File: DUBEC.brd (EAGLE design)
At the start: 40 x 21.4 mm, 72 parts

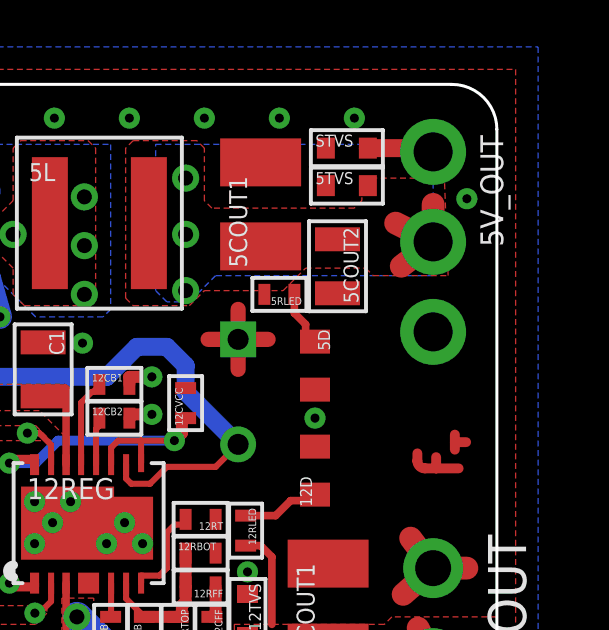
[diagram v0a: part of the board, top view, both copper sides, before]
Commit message: Tweaks
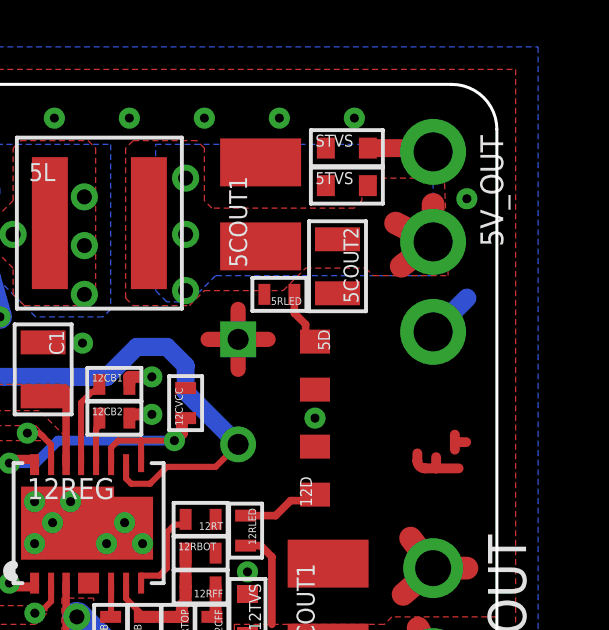
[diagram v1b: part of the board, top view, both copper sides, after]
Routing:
- net GND: track 34.1 -> 35.7 mm
- net 5V: track 44.4 -> 43.5 mm
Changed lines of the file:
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@@
 <grid distance="0.125" unitdist="mm" unit="mm" style="lines" multiple="8" display="yes" altdistance="0.0625" altunitdist="mm" altunit="mm"/>
 <layers>
-<layer number="1" name="Top" color="2" fill="1" visible="yes" active="yes"/>
+<layer number="1" name="Top" color="2" fill="1" visible="no" active="yes"/>
 <layer number="2" name="Route2" color="9" fill="1" visible="no" active="yes"/>
 <layer number="3" name="Route3" color="4" fill="3" visible="no" active="no"/>
 <layer number="14" name="Route14" color="1" fill="6" visible="no" active="no"/>
-<layer number="15" name="Route15" color="14" fill="1" visible="yes" active="yes"/>
+<layer number="15" name="Route15" color="14" fill="1" visible="no" active="yes"/>
 <layer number="16" name="Bottom" color="5" fill="1" visible="yes" active="yes"/>
 <layer number="17" name="Pads" color="10" fill="1" visible="yes" active="yes"/>
@@
 <layer number="20" name="Dimension" color="15" fill="1" visible="yes" active="yes"/>
 <layer number="21" name="tPlace" color="15" fill="1" visible="no" active="yes"/>
-<layer number="22" name="bPlace" color="7" fill="1" visible="no" active="yes"/>
-<layer number="23" name="tOrigins" color="15" fill="1" visible="yes" active="yes"/>
+<layer number="22" name="bPlace" color="7" fill="1" visible="yes" active="yes"/>
+<layer number="23" name="tOrigins" color="15" fill="1" visible="no" active="yes"/>
 <layer number="24" name="bOrigins" color="15" fill="1" visible="yes" active="yes"/>
 <layer number="25" name="tNames" color="7" fill="1" visible="no" active="yes"/>
@@
 <layer number="27" name="tValues" color="7" fill="1" visible="no" active="yes"/>
 <layer number="28" name="bValues" color="7" fill="1" visible="no" active="yes"/>
-<layer number="29" name="tStop" color="4" fill="1" visible="yes" active="yes"/>
+<layer number="29" name="tStop" color="4" fill="1" visible="no" active="yes"/>
 <layer number="30" name="bStop" color="7" fill="6" visible="yes" active="yes"/>
-<layer number="31" name="tCream" color="7" fill="4" visible="yes" active="yes"/>
+<layer number="31" name="tCream" color="7" fill="4" visible="no" active="yes"/>
 <layer number="32" name="bCream" color="7" fill="5" visible="yes" active="yes"/>
-<layer number="33" name="tFinish" color="6" fill="3" visible="yes" active="yes"/>
+<layer number="33" name="tFinish" color="6" fill="3" visible="no" active="yes"/>
 <layer number="34" name="bFinish" color="6" fill="6" visible="yes" active="yes"/>
-<layer number="35" name="tGlue" color="7" fill="4" visible="yes" active="yes"/>
+<layer number="35" name="tGlue" color="7" fill="4" visible="no" active="yes"/>
 <layer number="36" name="bGlue" color="7" fill="5" visible="yes" active="yes"/>
-<layer number="37" name="tTest" color="7" fill="1" visible="yes" active="yes"/>
+<layer number="37" name="tTest" color="7" fill="1" visible="no" active="yes"/>
 <layer number="38" name="bTest" color="7" fill="1" visible="yes" active="yes"/>
-<layer number="39" name="tKeepout" color="4" fill="11" visible="yes" active="yes"/>
+<layer number="39" name="tKeepout" color="4" fill="11" visible="no" active="yes"/>
 <layer number="40" name="bKeepout" color="1" fill="11" visible="yes" active="yes"/>
-<layer number="41" name="tRestrict" color="14" fill="10" visible="yes" active="yes"/>
+<layer number="41" name="tRestrict" color="14" fill="10" visible="no" active="yes"/>
 <layer number="42" name="bRestrict" color="1" fill="10" visible="yes" active="yes"/>
 <layer number="43" name="vRestrict" color="2" fill="10" visible="no" active="yes"/>
 <layer number="44" name="Drills" color="7" fill="1" visible="no" active="yes"/>
-<layer number="45" name="Holes" color="7" fill="1" visible="no" active="yes"/>
+<layer number="45" name="Holes" color="7" fill="1" visible="yes" active="yes"/>
 <layer number="46" name="Milling" color="3" fill="1" visible="no" active="yes"/>
 <layer number="47" name="Measures" color="7" fill="1" visible="yes" active="yes"/>
-<layer number="48" name="Document" color="7" fill="1" visible="no" active="yes"/>
+<layer number="48" name="Document" color="7" fill="1" visible="yes" active="yes"/>
 <layer number="49" name="Reference" color="7" fill="1" visible="no" active="yes"/>
 <layer number="50" name="dxf" color="7" fill="1" visible="no" active="no"/>
 <layer number="51" name="tDocu" color="7" fill="1" visible="no" active="yes"/>
-<layer number="52" name="bDocu" color="7" fill="1" visible="no" active="yes"/>
+<layer number="52" name="bDocu" color="7" fill="1" visible="yes" active="yes"/>
 <layer number="53" name="tGND_GNDA" color="7" fill="9" visible="no" active="no"/>
 <layer number="54" name="bGND_GNDA" color="1" fill="9" visible="no" active="no"/>
@@
 <layer number="100" name="Muster" color="7" fill="1" visible="no" active="no"/>
 <layer number="101" name="Patch_Top" color="12" fill="4" visible="no" active="yes"/>
-<layer number="102" name="tPolarity" color="7" fill="1" visible="yes" active="yes"/>
+<layer number="102" name="tPolarity" color="7" fill="1" visible="no" active="yes"/>
 <layer number="103" name="tMap" color="7" fill="1" visible="no" active="yes"/>
 <layer number="104" name="Name" color="16" fill="1" visible="no" active="yes"/>
-<layer number="105" name="tPlate" color="7" fill="1" visible="yes" active="yes"/>
+<layer number="105" name="tPlate" color="7" fill="1" visible="no" active="yes"/>
 <layer number="106" name="bPlate" color="7" fill="1" visible="no" active="yes"/>
-<layer number="107" name="tLabels" color="15" fill="1" visible="yes" active="yes"/>
+<layer number="107" name="tLabels" color="15" fill="1" visible="no" active="yes"/>
 <layer number="108" name="tplace-old" color="10" fill="1" visible="no" active="yes"/>
 <layer number="109" name="ref-old" color="11" fill="1" visible="no" active="yes"/>
@@
 <wire x1="36.5" y1="1" x2="36.75" y2="0.75" width="0.254" layer="1"/>
 <wire x1="36.75" y1="0.75" x2="38.75" y2="0.75" width="0.254" layer="1"/>
+<wire x1="37.875" y1="13.125" x2="39" y2="14.25" width="0.635" layer="16"/>
 </signal>
 <signal name="12V">
@@
 <wire x1="15.75" y1="16.75" x2="15.75" y2="17.5" width="0.4" layer="1"/>
 <via x="29.625" y="14.5" extent="1-16" drill="0.5"/>
-<wire x1="29.625" y1="14.5" x2="29.625" y2="16.375" width="1.016" layer="15"/>
+<wire x1="29.625" y1="14.5" x2="29.625" y2="16.125" width="1.016" layer="15"/>
+<wire x1="29.625" y1="16.125" x2="29.625" y2="16.375" width="1.016" layer="15"/>
 <wire x1="29.625" y1="16.375" x2="29.625" y2="18.25" width="1.016" layer="15"/>
 <via x="29.625" y="16.375" extent="1-16" drill="0.5"/>
@@
 <via x="17.25" y="13" extent="1-16" drill="0.3"/>
 <wire x1="17.25" y1="13" x2="17.25" y2="14.875" width="0.3302" layer="15"/>
-<wire x1="29.625" y1="18.25" x2="35.75" y2="18.25" width="1" layer="15"/>
-<wire x1="35.75" y1="18.25" x2="37.875" y2="16.125" width="1" layer="15"/>
 <wire x1="16.625" y1="12.875" x2="16.75" y2="13" width="0.4" layer="1"/>
 <wire x1="16.75" y1="13" x2="17.25" y2="13" width="0.4" layer="1"/>
 <contactref element="5COUT2" pad="1"/>
 <contactref element="5COUT1" pad="A"/>
+<wire x1="37.875" y1="16.125" x2="29.625" y2="16.125" width="1.016" layer="15"/>
 </signal>
 <signal name="12V_FB">
@@
 <wire x1="14" y1="16.125" x2="14.625" y2="16.125" width="0.4" layer="1"/>
 <wire x1="2" y1="10.125" x2="4.5" y2="10.125" width="0.3302" layer="15"/>
-<wire x1="4.5" y1="10.125" x2="8.875" y2="14.5" width="0.3302" layer="15"/>
-<wire x1="8.875" y1="14.5" x2="13" y2="14.5" width="0.3302" layer="15"/>
-<wire x1="13" y1="14.5" x2="14.625" y2="16.125" width="0.3302" layer="15"/>
+<wire x1="4.5" y1="10.125" x2="8.5" y2="14.125" width="0.3302" layer="15"/>
+<wire x1="8.5" y1="14.125" x2="12.625" y2="14.125" width="0.3302" layer="15"/>
+<wire x1="12.625" y1="14.125" x2="14.625" y2="16.125" width="0.3302" layer="15"/>
 </signal>
 <signal name="GATE_MAIN_B" class="2">

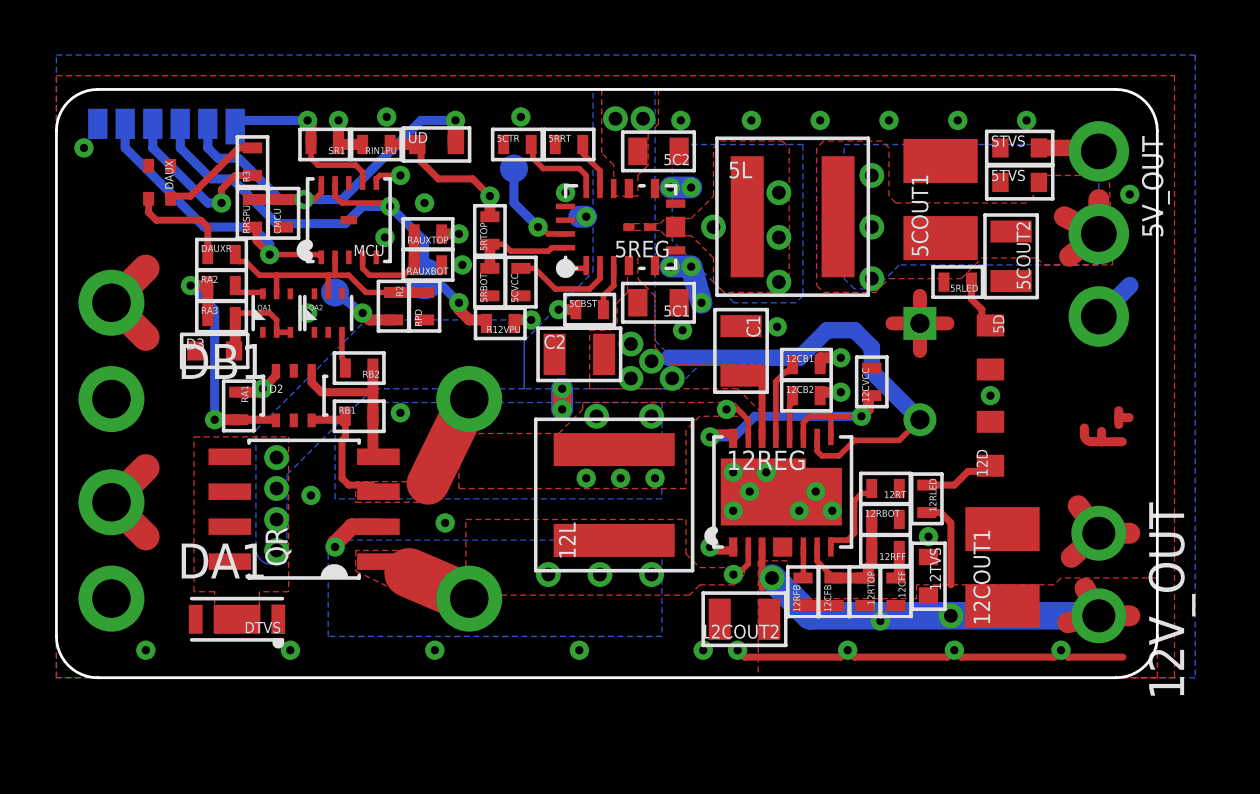
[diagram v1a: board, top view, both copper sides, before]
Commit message: Tweaks
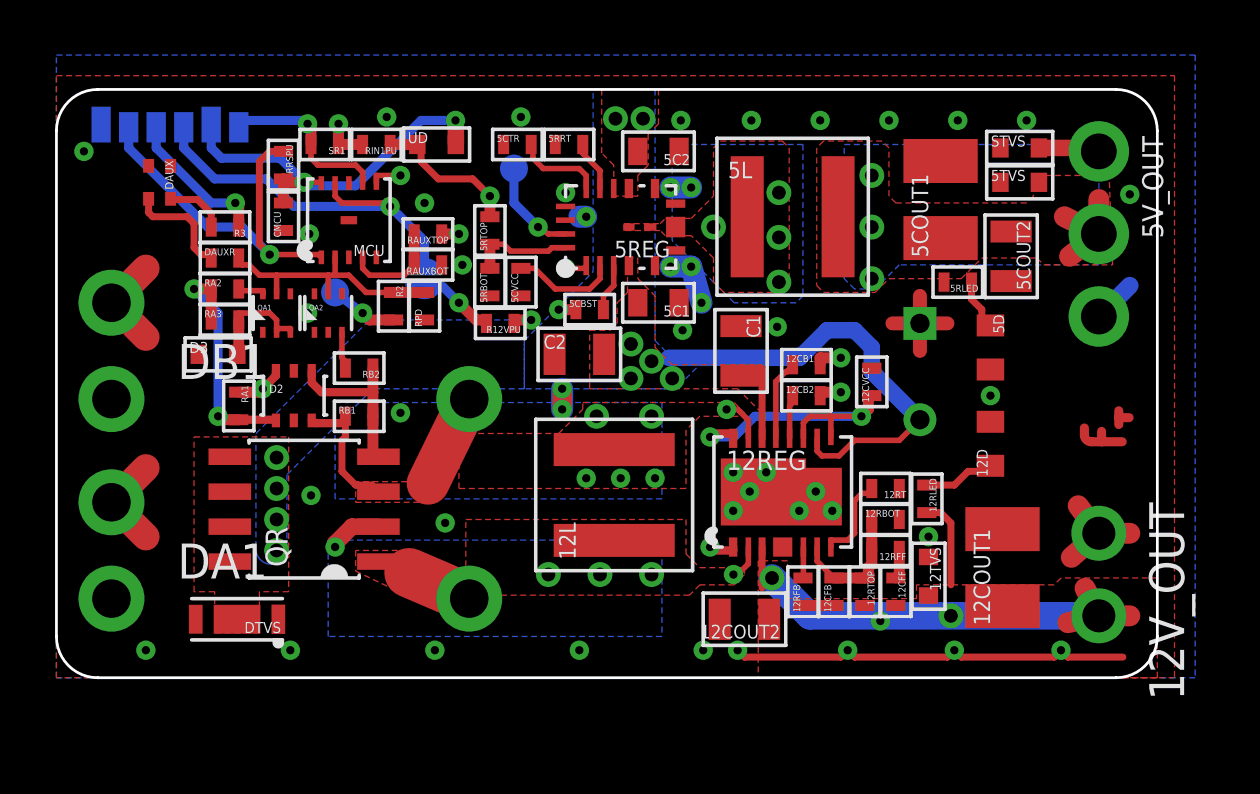
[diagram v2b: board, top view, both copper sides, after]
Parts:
- moved R3 2.58 mm to (6.12, 16.4), turned to 180 degrees
- moved RRSPU 2.08 mm to (8.25, 18.6), turned to 270 degrees
- moved AVRISP 0.18 mm to (4.12, 20.0)
- moved D3 0.18 mm to (5.88, 11.8)
- moved DAUXR 0.18 mm to (6.12, 15.2)
- moved RA2 0.18 mm to (6.12, 14.1)
- moved RA3 0.18 mm to (6.12, 13.0)
- moved CMCU 0.12 mm to (8.25, 16.8)
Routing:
- net RESET: track 11.1 -> 14.0 mm
- net LED_RED: track 3.74 -> 2.19 mm
- net 5V_MCU: track 15.7 -> 14.5 mm
- net SCK: track 15.4 -> 14.6 mm
- net MOSI: track 14.0 -> 13.5 mm
